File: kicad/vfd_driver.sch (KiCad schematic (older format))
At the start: 40 parts, among them CON1 AVR-ISP-6, J1 PWR, J6 MH, J7 MH, J8 MH, J9 MH, U1 ATTINY2313-20SU, U10 74HC595, U11 74HC595, U12 74HC595, U13 74HC595, U14 ULN2803A, U15 ULN2803A, U16 ULN2003, U17 ULN2003, U18 LM1117-3.3, U2 74HC595, U3 74HC595, U4 74HC595, U5 74HC595, U6 ULN2803A, U7 ULN2003, U8 ULN2003, U9 ULN2003

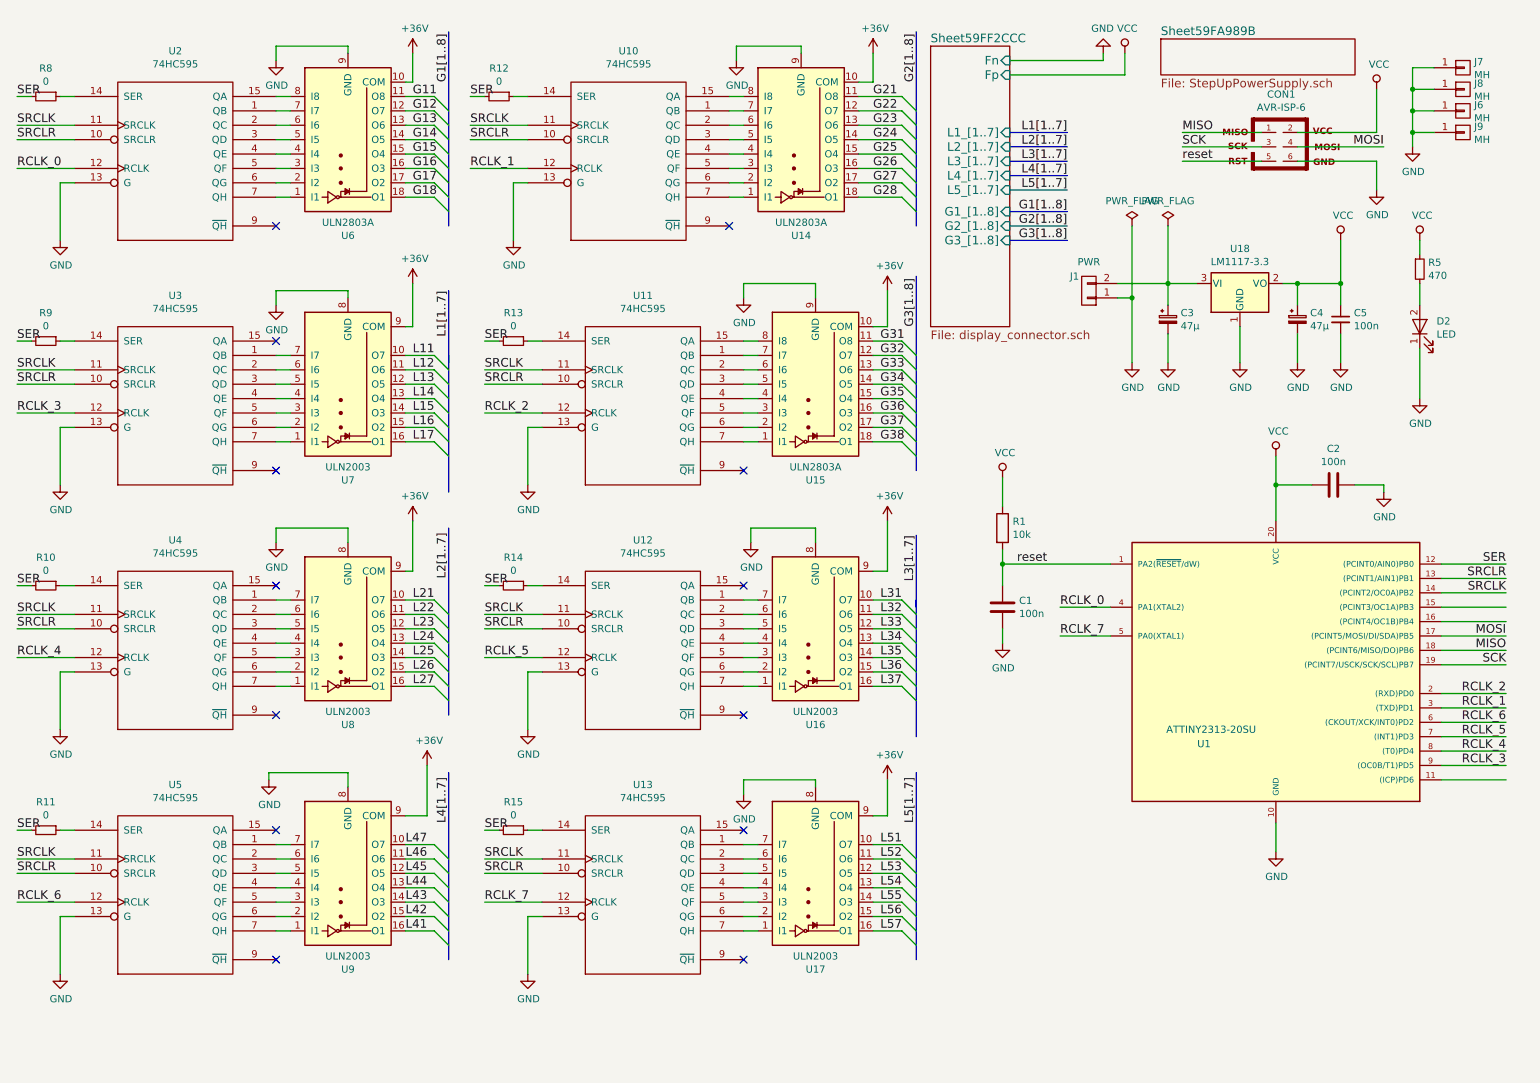
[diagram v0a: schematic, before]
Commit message: routing
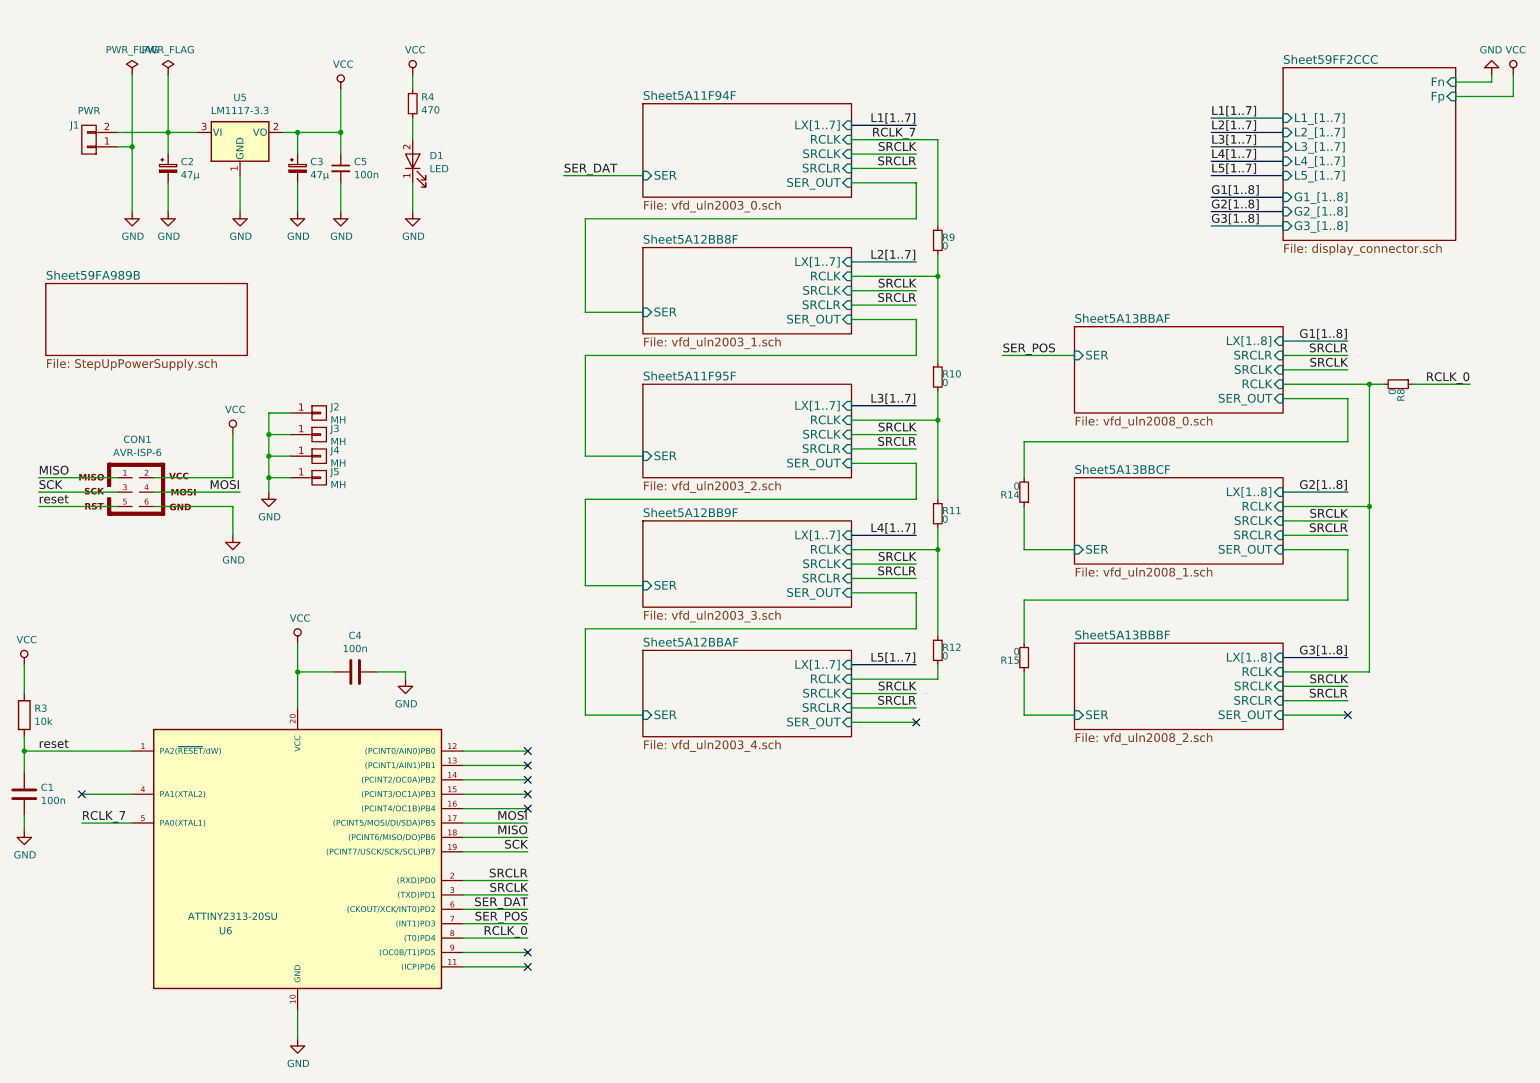
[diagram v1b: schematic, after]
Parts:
- removed R13: 0, Resistors_SMD:R_1206, symbol R_Small
- removed U10, U11, U12, U13, U2, U3, U4, U5: 74HC595, Housings_SOIC:SOIC-16_3.9x9.9mm_Pitch1.27mm, symbol 74HC595
- removed U14, U15, U6: ULN2803A, Housings_SOIC:SOIC-18W_7.5x11.6mm_Pitch1.27mm, symbol ULN2803A
- removed U16, U17, U7, U8, U9: ULN2003, Housings_SOIC:SOIC-16_3.9x9.9mm_Pitch1.27mm, symbol ULN2003
- renumbered C3 to C2, C4 to C3, C2 to C4, D2 to D1, J7 to J2, J8 to J3, J6 to J4, J9 to J5, R1 to R3, R5 to R4, U18 to U5, U1 to U6
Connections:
- net RCLK_1 is gone; now on net SRCLK: U6.3 ((TXD)PD1)
- net RCLK_2 is gone; now on net SRCLR: U6.2 ((RXD)PD0)
- net RCLK_4 is gone; now on net RCLK_0: U6.8 ((T0)PD4)
- net RCLK_0: now also R8.1; no longer U6.4 (PA1(XTAL2))
- net RCLK_7: now also R9.1
- net SRCLK: no longer U6.14 ((PCINT2/OC0A)PB2)
- net SRCLR: no longer U6.13 ((PCINT1/AIN1)PB1)
- net Sheet5A13BBBF/SER: now reaches R15.1
- net Sheet5A11F95F/RCLK: now reaches R11.1
- net Sheet5A11F95F/RCLK: now also R10.2
- net Sheet5A13BBCF/SER: now reaches R14.1
- net Sheet5A12BB8F/RCLK: now reaches R10.1
- net Sheet5A12BB8F/RCLK: now also R9.2
- net Sheet5A12BB9F/RCLK: now reaches R12.1
- net Sheet5A12BB9F/RCLK: now also R11.2
- net RCLK_3: no longer names the net of U6.9 ((OC0B/T1)PD5)
- net RCLK_5 renamed SER_POS
- net RCLK_6 renamed SER_DAT
- removed net SER: R10.2, R11.2, R12.2, R14.2, R15.2, R8.2, R9.2, U6.12 ((PCINT0/AIN0)PB0)
- new net Sheet5A12BBAF/RCLK: R12.2
- new net Sheet5A13BBAF/RCLK: R8.2
- new net Sheet5A13BBAF/SER_OUT: R14.2
- new net Sheet5A13BBCF/SER_OUT: R15.2
- no-connect marks 13 -> 10
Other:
- moved on the sheet: C1, C2, C3, C4, C5, CON1, D1, J1, J2, J3, J4, J5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
